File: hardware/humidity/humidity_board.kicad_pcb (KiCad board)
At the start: 2 copper layers, 100 x 20 mm, 23 parts, among them IC1 ATMEGA88-A, J1 RJ45, P1 ISP, P2 UART, SW1 SW_RESET, U1 ST485, U2 HYT271, m3_loch VAL**

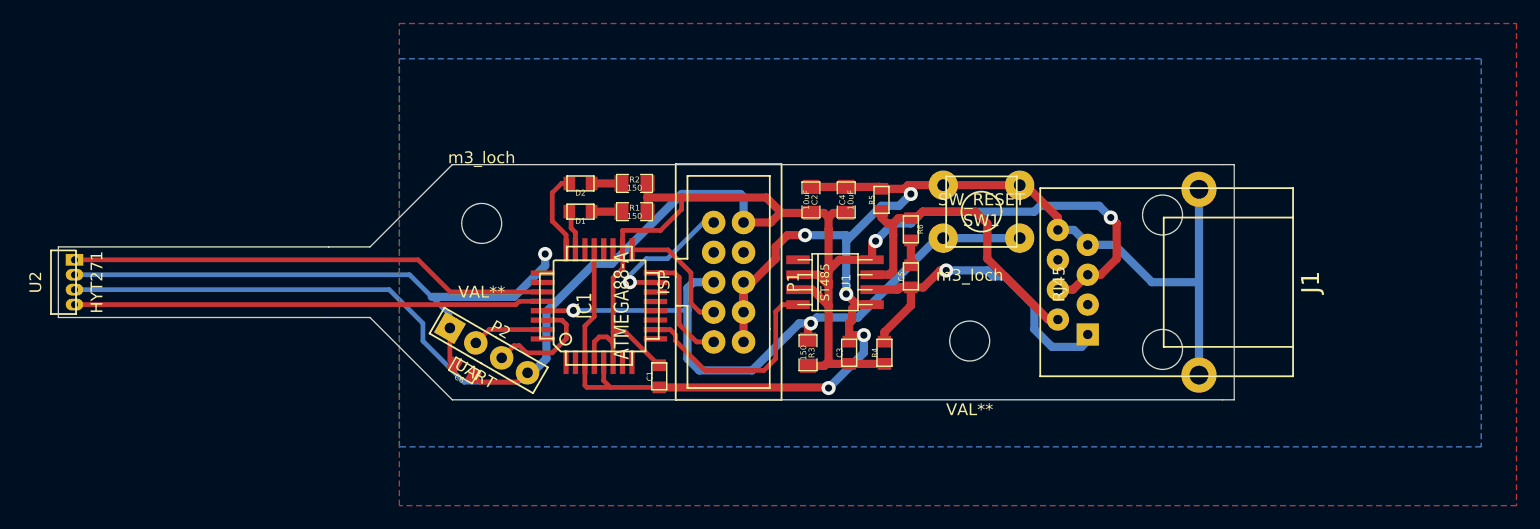
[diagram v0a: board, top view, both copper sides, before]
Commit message: finalized boards for production
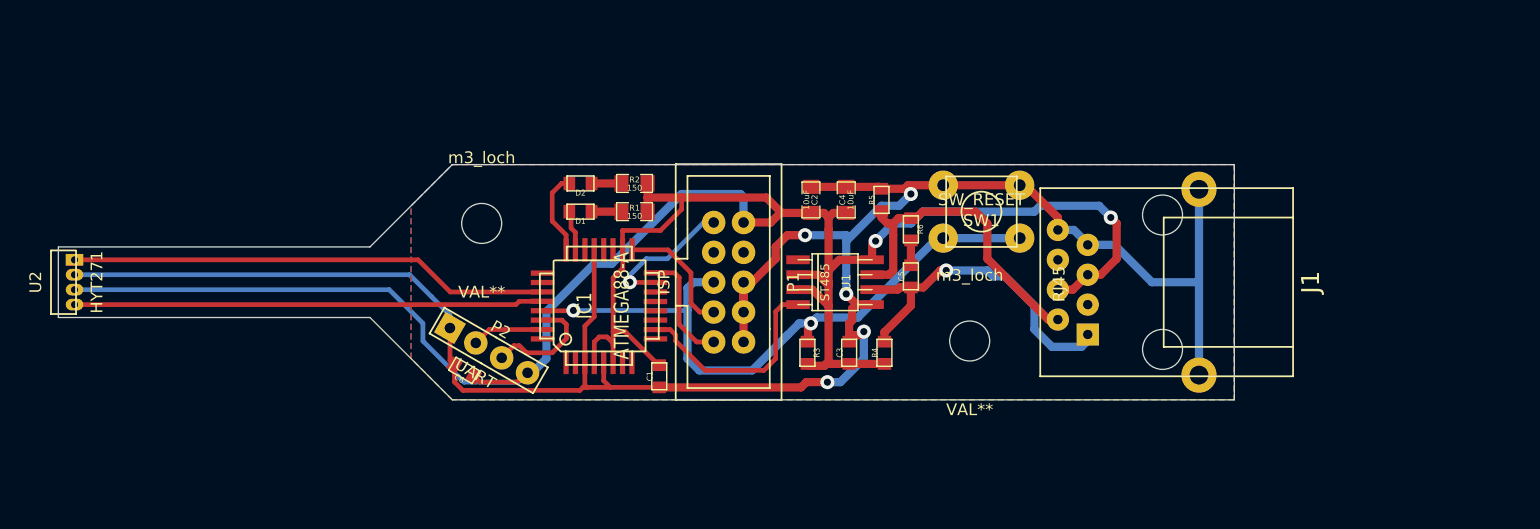
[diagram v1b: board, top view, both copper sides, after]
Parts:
- R3: value 150 -> 10k; footprint SM0805_big -> SM0603_big
- moved R3 0.05 mm to (163.7, 102.0)
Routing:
- net GND: track 182.6 -> 184.4 mm, vias 6 -> 5
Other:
- outline, holes or cut-outs redrawn
